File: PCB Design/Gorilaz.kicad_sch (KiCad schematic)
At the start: 44 parts, among them J1 Conn_01x13, J2 Conn_01x13, J3 Conn_01x13, J4 Conn_01x13, J5 HRO_TYPE-C-31-M-14, J6 Battery, J7 Conn_01x13, J8 Conn_01x13, SW1 SW_DPST_x2, SW4 RST, U1 SRV05-4, U10 MAX17048, U3 BQ24075, U4 DW01A, U5 FS8205, U8 nRF52840_moko_mk08

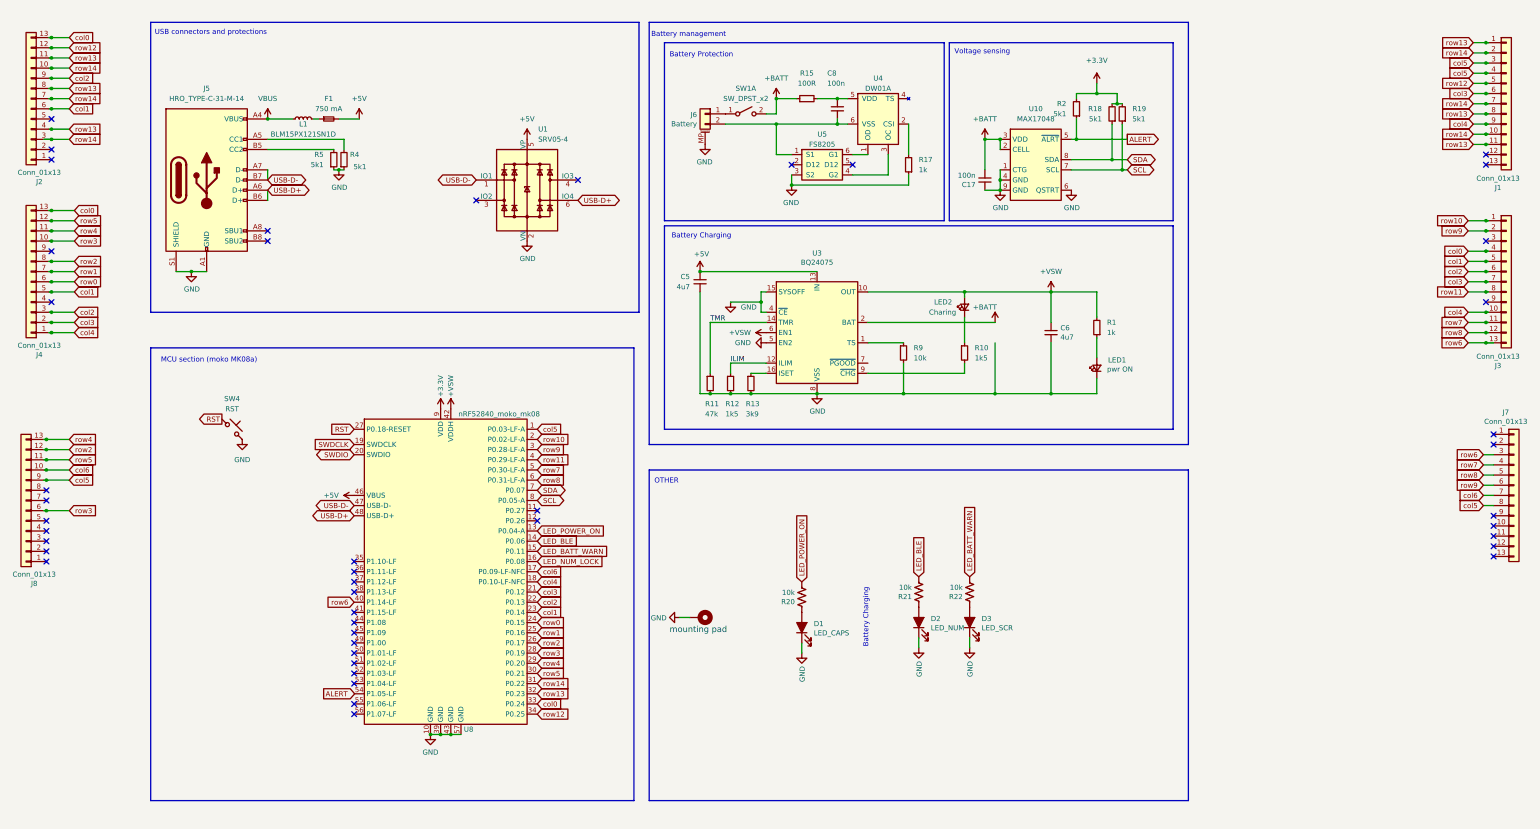
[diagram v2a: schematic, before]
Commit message: render update
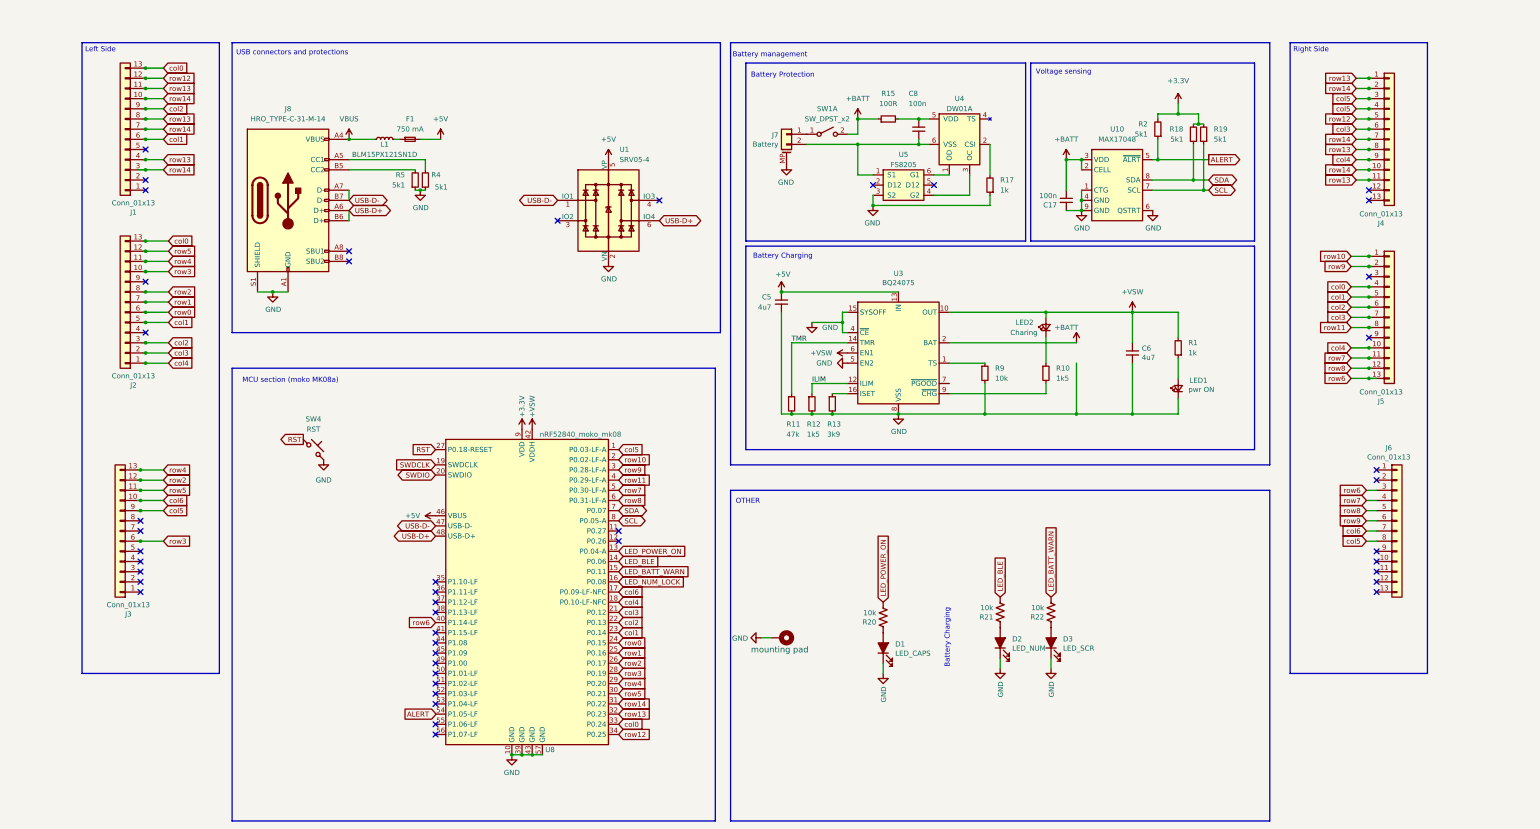
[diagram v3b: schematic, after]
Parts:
- renumbered J2 to J1, J4 to J2, J8 to J3, J1 to J4, J3 to J5, J7 to J6, J6 to J7, J5 to J8
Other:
- note added: "Left Side"
- note added: "Right Side"
- moved on the sheet: C17, C5, C6, C8, D1, D2, D3, F1, J1, J2, J3, J4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
